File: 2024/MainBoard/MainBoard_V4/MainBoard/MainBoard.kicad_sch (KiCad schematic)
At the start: 96 parts, among them J1 Raspberry_Pi_2_3, J10 ADC3, J11 ADC2, J12 ADC2, J13 Drib, J14 UART, J15 TFT3, J16 CAN_CON, J2 fan, J3 USB_C_Receptacle_USB2.0_16P, J4 CAN_CON, J5 MOLEX MINISPOX, J6 Debug, J7 ADC0, J8 ADC1, J9 ADC2, Q1 NMOS, Q2 PMOS, Q3 PMOS, SW1 SW_MEC_5E, SW2 SW_MEC_5E, SW3 SW_MEC_5E, SW4 SW_Wuerth_450301014042, U1 STM32F446RETx, U2 CH340E, U3 MOUDLE-SEEEDUINO-XIAO, U7 AZ1117-3.3, U8 MAX3051, Y1 CSTNE16M0V530000R0

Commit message: 部品をおいた
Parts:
- J10, J11, J12, J7, J8, J9: footprint Connector_JST:JST_XH_S3B-XH-A_1x03_P2.50mm_Horizontal -> Connector_JST:JST_PH_B3B-PH-K_1x03_P2.00mm_Vertical
- LS1: footprint PKLCS1212E4001-R1:SPKR_PKLCS1212E4001-R1 -> MainBoard:SPKR_PKLCS1212E4001-R1
- ROTSW1: footprint (none) -> Button_Switch_THT:Nidec_Copal_SH-7010C
- U5: footprint Connector_PinHeader_2.54mm:PinHeader_1x05_P2.54mm_Vertical -> Connector_PinHeader_2.54mm:PinHeader_1x04_P2.54mm_Vertical
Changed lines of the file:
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@@
       (effects (font (size 1.27 1.27)))
     )
-    (property "Footprint" "Connector_PinHeader_2.54mm:PinHeader_1x05_P2.54mm_Vertical" (at 222.25 240.03 0)
+    (property "Footprint" "Connector_PinHeader_2.54mm:PinHeader_1x04_P2.54mm_Vertical" (at 222.25 240.03 0)
       (effects (font (size 1.27 1.27)) hide)
     )
@@
       (effects (font (size 1.27 1.27)) (justify left) hide)
     )
-    (property "Footprint" "PKLCS1212E4001-R1:SPKR_PKLCS1212E4001-R1" (at 398.78 52.07 0)
+    (property "Footprint" "MainBoard:SPKR_PKLCS1212E4001-R1" (at 398.78 52.07 0)
       (effects (font (size 1.27 1.27)) (justify bottom) hide)
     )
@@
       (effects (font (size 1.27 1.27)) (justify left))
     )
-    (property "Footprint" "Connector_JST:JST_XH_S3B-XH-A_1x03_P2.50mm_Horizontal" (at 483.87 119.38 0)
+    (property "Footprint" "Connector_JST:JST_PH_B3B-PH-K_1x03_P2.00mm_Vertical" (at 483.87 119.38 0)
       (effects (font (size 1.27 1.27)) hide)
     )
@@
       (effects (font (size 1.27 1.27)) (justify left))
     )
-    (property "Footprint" "Connector_JST:JST_XH_S3B-XH-A_1x03_P2.50mm_Horizontal" (at 483.87 99.06 0)
+    (property "Footprint" "Connector_JST:JST_PH_B3B-PH-K_1x03_P2.00mm_Vertical" (at 483.87 99.06 0)
       (effects (font (size 1.27 1.27)) hide)
     )
@@
       (effects (font (size 1.27 1.27)) (justify left))
     )
-    (property "Footprint" "Connector_JST:JST_XH_S3B-XH-A_1x03_P2.50mm_Horizontal" (at 514.35 119.38 0)
+    (property "Footprint" "Connector_JST:JST_PH_B3B-PH-K_1x03_P2.00mm_Vertical" (at 514.35 119.38 0)
       (effects (font (size 1.27 1.27)) hide)
     )
@@
       (effects (font (size 1.27 1.27)) (justify left))
     )
-    (property "Footprint" "Connector_JST:JST_XH_S3B-XH-A_1x03_P2.50mm_Horizontal" (at 483.87 78.74 0)
+    (property "Footprint" "Connector_JST:JST_PH_B3B-PH-K_1x03_P2.00mm_Vertical" (at 483.87 78.74 0)
       (effects (font (size 1.27 1.27)) hide)
     )
@@
       (effects (font (size 1.27 1.27)))
     )
-    (property "Footprint" "" (at 133.35 237.49 0)
+    (property "Footprint" "Button_Switch_THT:Nidec_Copal_SH-7010C" (at 133.35 237.49 0)
       (effects (font (size 1.27 1.27)) (justify left) hide)
     )
@@
       (effects (font (size 1.27 1.27)) (justify left))
     )
-    (property "Footprint" "Connector_JST:JST_XH_S3B-XH-A_1x03_P2.50mm_Horizontal" (at 514.35 78.74 0)
+    (property "Footprint" "Connector_JST:JST_PH_B3B-PH-K_1x03_P2.00mm_Vertical" (at 514.35 78.74 0)
       (effects (font (size 1.27 1.27)) hide)
     )
@@
       (effects (font (size 1.27 1.27)) (justify left))
     )
-    (property "Footprint" "Connector_JST:JST_XH_S3B-XH-A_1x03_P2.50mm_Horizontal" (at 514.35 99.06 0)
+    (property "Footprint" "Connector_JST:JST_PH_B3B-PH-K_1x03_P2.00mm_Vertical" (at 514.35 99.06 0)
       (effects (font (size 1.27 1.27)) hide)
     )

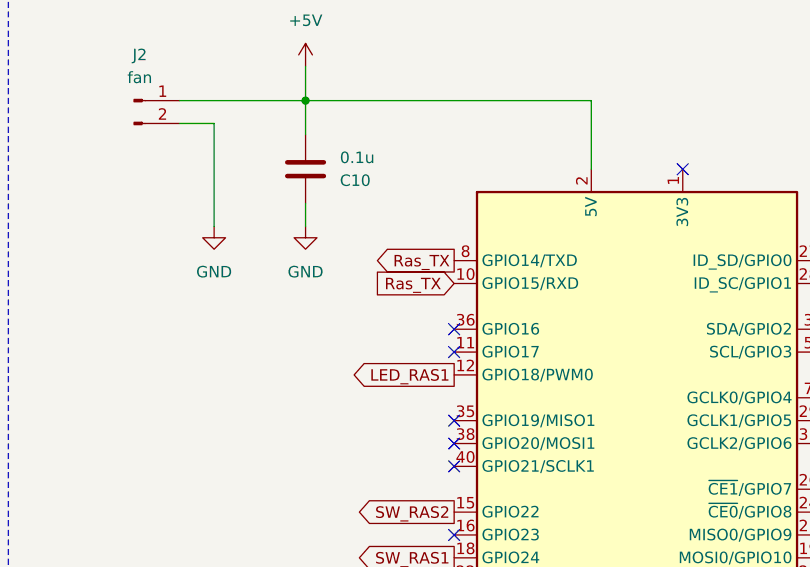
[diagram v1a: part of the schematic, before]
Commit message: わくぎめ
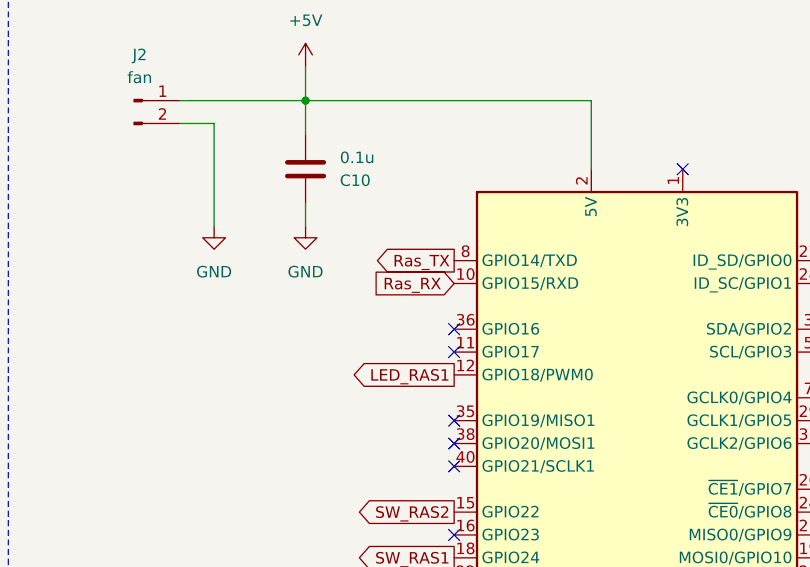
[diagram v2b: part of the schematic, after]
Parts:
- J10, J11, J12, J7, J8, J9: footprint Connector_JST:JST_PH_B3B-PH-K_1x03_P2.00mm_Vertical -> Connector_JST:JST_PH_S3B-PH-K_1x03_P2.00mm_Horizontal
- J5: footprint Connector_Molex:Molex_SPOX_5267-06A_1x06_P2.50mm_Vertical -> Connector_Molex:Molex_SPOX_5268-06A_1x06_P2.50mm_Horizontal
- SW2, SW3: footprint Button_Switch_THT:SW_PUSH_6mm -> MainBoard:SW_SKRPACE010
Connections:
- net Ras_RX: now also J1.10 (GPIO15/RXD)
- net Ras_TX: no longer J1.10 (GPIO15/RXD)
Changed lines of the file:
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@@
     )
   )
-  (global_label "Ras_TX" (shape input) (at 74.93 226.06 180) (fields_autoplaced)
+  (global_label "Ras_RX" (shape input) (at 74.93 226.06 180) (fields_autoplaced)
     (effects (font (size 1.27 1.27)) (justify right))
-    (property "Intersheetrefs" "${INTERSHEET_REFS}" (at 65.5788 226.06 0)
+    (property "Intersheetrefs" "${INTERSHEET_REFS}" (at 65.0506 226.06 0)
       (effects (font (size 1.27 1.27)) (justify right) hide)
     )
@@
       (effects (font (size 1.27 1.27)))
     )
-    (property "Footprint" "Button_Switch_THT:SW_PUSH_6mm" (at 138.43 262.89 0)
+    (property "Footprint" "MainBoard:SW_SKRPACE010" (at 138.43 262.89 0)
       (effects (font (size 1.27 1.27)) hide)
     )
@@
       (effects (font (size 1.27 1.27)) (justify left))
     )
-    (property "Footprint" "Connector_JST:JST_PH_B3B-PH-K_1x03_P2.00mm_Vertical" (at 483.87 119.38 0)
+    (property "Footprint" "Connector_JST:JST_PH_S3B-PH-K_1x03_P2.00mm_Horizontal" (at 483.87 119.38 0)
       (effects (font (size 1.27 1.27)) hide)
     )
@@
       (effects (font (size 1.27 1.27)) (justify left))
     )
-    (property "Footprint" "Connector_Molex:Molex_SPOX_5267-06A_1x06_P2.50mm_Vertical" (at 486.41 55.88 0)
+    (property "Footprint" "Connector_Molex:Molex_SPOX_5268-06A_1x06_P2.50mm_Horizontal" (at 486.41 55.88 0)
       (effects (font (size 1.27 1.27)) hide)
     )
@@
       (effects (font (size 1.27 1.27)) (justify left))
     )
-    (property "Footprint" "Connector_JST:JST_PH_B3B-PH-K_1x03_P2.00mm_Vertical" (at 483.87 99.06 0)
+    (property "Footprint" "Connector_JST:JST_PH_S3B-PH-K_1x03_P2.00mm_Horizontal" (at 483.87 99.06 0)
       (effects (font (size 1.27 1.27)) hide)
     )
@@
       (effects (font (size 1.27 1.27)) (justify left))
     )
-    (property "Footprint" "Connector_JST:JST_PH_B3B-PH-K_1x03_P2.00mm_Vertical" (at 514.35 119.38 0)
+    (property "Footprint" "Connector_JST:JST_PH_S3B-PH-K_1x03_P2.00mm_Horizontal" (at 514.35 119.38 0)
       (effects (font (size 1.27 1.27)) hide)
     )
@@
       (effects (font (size 1.27 1.27)) (justify left))
     )
-    (property "Footprint" "Connector_JST:JST_PH_B3B-PH-K_1x03_P2.00mm_Vertical" (at 483.87 78.74 0)
+    (property "Footprint" "Connector_JST:JST_PH_S3B-PH-K_1x03_P2.00mm_Horizontal" (at 483.87 78.74 0)
       (effects (font (size 1.27 1.27)) hide)
     )
@@
       (effects (font (size 1.27 1.27)) (justify left))
     )
-    (property "Footprint" "Connector_JST:JST_PH_B3B-PH-K_1x03_P2.00mm_Vertical" (at 514.35 78.74 0)
+    (property "Footprint" "Connector_JST:JST_PH_S3B-PH-K_1x03_P2.00mm_Horizontal" (at 514.35 78.74 0)
       (effects (font (size 1.27 1.27)) hide)
     )
@@
       (effects (font (size 1.27 1.27)) (justify left))
     )
-    (property "Footprint" "Connector_JST:JST_PH_B3B-PH-K_1x03_P2.00mm_Vertical" (at 514.35 99.06 0)
+    (property "Footprint" "Connector_JST:JST_PH_S3B-PH-K_1x03_P2.00mm_Horizontal" (at 514.35 99.06 0)
       (effects (font (size 1.27 1.27)) hide)
     )
@@
       (effects (font (size 1.27 1.27)))
     )
-    (property "Footprint" "Button_Switch_THT:SW_PUSH_6mm" (at 138.43 246.38 0)
+    (property "Footprint" "MainBoard:SW_SKRPACE010" (at 138.43 246.38 0)
       (effects (font (size 1.27 1.27)) hide)
     )

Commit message: 途中経過
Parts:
- D5: footprint Diode_THT:D_DO-35_SOD27_P7.62mm_Horizontal -> Diode_SMD:D_SOD-123
- Q2, Q3: footprint (none) -> Package_TO_SOT_SMD:SOT-23
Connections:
- net UART_RX is gone; now on net UART1_TX: J6.1 (Pin_1)
- net UART_TX is gone; now on net UART1_RX: J6.2 (Pin_2)
- net VDD is gone; now on net +3.3V: J6.6 (Pin_6)
- net CANH: now also J16.2 (Pin_2); no longer J16.1 (Pin_1)
- net CANL: now also J16.1 (Pin_1); no longer J16.2 (Pin_2)
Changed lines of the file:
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@@
+    )
+  )
+  (global_label "CANH" (shape bidirectional) (at 509.27 50.8 180) (fields_autoplaced)
+    (effects (font (size 1.27 1.27)) (justify right))
+    (property "Intersheetrefs" "${INTERSHEET_REFS}" (at 500.1539 50.8 0)
+      (effects (font (size 1.27 1.27)) (justify right) hide)
     )
   )
@@
     )
   )
-  (global_label "UART_RX" (shape input) (at 45.72 139.7 0) (fields_autoplaced)
-    (effects (font (size 1.27 1.27)) (justify left))
-    (property "Intersheetrefs" "${INTERSHEET_REFS}" (at 56.1692 139.7 0)
-      (effects (font (size 1.27 1.27)) (justify left) hide)
-    )
-  )
   (global_label "LED_RAS1" (shape output) (at 495.3 184.15 180) (fields_autoplaced)
     (effects (font (size 1.27 1.27)) (justify right))
@@
     )
   )
-  (global_label "CANH" (shape bidirectional) (at 509.27 48.26 180) (fields_autoplaced)
-    (effects (font (size 1.27 1.27)) (justify right))
-    (property "Intersheetrefs" "${INTERSHEET_REFS}" (at 500.1539 48.26 0)
-      (effects (font (size 1.27 1.27)) (justify right) hide)
-    )
-  )
   (global_label "LED1" (shape output) (at 533.4 171.45 180) (fields_autoplaced)
     (effects (font (size 1.27 1.27)) (justify right))
@@
     )
   )
-  (global_label "UART_TX" (shape output) (at 45.72 142.24 0) (fields_autoplaced)
-    (effects (font (size 1.27 1.27)) (justify left))
-    (property "Intersheetrefs" "${INTERSHEET_REFS}" (at 56.1692 142.24 0)
-      (effects (font (size 1.27 1.27)) (justify left) hide)
-    )
-  )
   (global_label "CANL" (shape bidirectional) (at 509.27 60.96 180) (fields_autoplaced)
     (effects (font (size 1.27 1.27)) (justify right))
@@
     )
   )
-  (global_label "CANL" (shape bidirectional) (at 509.27 50.8 180) (fields_autoplaced)
-    (effects (font (size 1.27 1.27)) (justify right))
-    (property "Intersheetrefs" "${INTERSHEET_REFS}" (at 500.4563 50.8 0)
-      (effects (font (size 1.27 1.27)) (justify right) hide)
-    )
-  )
   (global_label "I2C_SCL" (shape bidirectional) (at 293.37 132.08 180) (fields_autoplaced)
     (effects (font (size 1.27 1.27)) (justify right))
@@
     )
   )
+  (global_label "USB_RX" (shape input) (at 45.72 139.7 0) (fields_autoplaced)
+    (effects (font (size 1.27 1.27)) (justify left))
+    (property "Intersheetrefs" "${INTERSHEET_REFS}" (at 55.0712 139.7 0)
+      (effects (font (size 1.27 1.27)) (justify left) hide)
+    )
+  )
+  (global_label "USB_TX" (shape output) (at 45.72 142.24 0) (fields_autoplaced)
+    (effects (font (size 1.27 1.27)) (justify left))
+    (property "Intersheetrefs" "${INTERSHEET_REFS}" (at 55.0712 142.24 0)
+      (effects (font (size 1.27 1.27)) (justify left) hide)
+    )
+  )
   (global_label "UART4_TX" (shape output) (at 203.2 35.56 180) (fields_autoplaced)
     (effects (font (size 1.27 1.27)) (justify right))
@@
     )
   )
+  (global_label "CANL" (shape bidirectional) (at 509.27 48.26 180) (fields_autoplaced)
+    (effects (font (size 1.27 1.27)) (justify right))
+    (property "Intersheetrefs" "${INTERSHEET_REFS}" (at 500.4563 48.26 0)
+      (effects (font (size 1.27 1.27)) (justify right) hide)
+    )
+  )
   (global_label "RAS_AUDIO" (shape output) (at 115.57 266.7 0) (fields_autoplaced)
     (effects (font (size 1.27 1.27)) (justify left))
@@
       (effects (font (size 1.27 1.27)))
     )
-    (property "Footprint" "" (at 191.77 69.85 0)
+    (property "Footprint" "Package_TO_SOT_SMD:SOT-23" (at 191.77 69.85 0)
       (effects (font (size 1.27 1.27)) hide)
     )
@@
     )
   )
-  (symbol (lib_id "power:VDD") (at 58.42 139.7 0) (unit 1)
-    (in_bom yes) (on_board yes) (dnp no)
-    (property "Reference" "#PWR064" (at 58.42 143.51 0)
-      (effects (font (size 1.27 1.27)) hide)
-    )
-    (property "Value" "VDD" (at 58.801 136.4488 0)
-      (effects (font (size 1.27 1.27)) (justify left))
-    )
-    (property "Footprint" "" (at 58.42 139.7 0)
-      (effects (font (size 1.27 1.27)) hide)
-    )
-    (property "Datasheet" "" (at 58.42 139.7 0)
-      (effects (font (size 1.27 1.27)) hide)
-    )
-    (pin "1")
-    (instances
-      (project "MainBoard"
-        (path "/0f1369eb-a284-48b8-a3ed-798a8062c1cf"
-          (reference "#PWR064") (unit 1)
-        )
-      )
-    )
-  )
   (symbol (lib_id "Device:LED") (at 527.05 201.93 90) (unit 1)
     (in_bom yes) (on_board yes) (dnp no)
@@
       (effects (font (size 1.27 1.27)))
     )
-    (property "Footprint" "" (at 186.69 69.85 0)
+    (property "Footprint" "Package_TO_SOT_SMD:SOT-23" (at 186.69 69.85 0)
       (effects (font (size 1.27 1.27)) hide)
     )
@@
     )
   )
+  (symbol (lib_id "power:+3.3V") (at 58.42 139.7 0) (unit 1)
+    (in_bom yes) (on_board yes) (dnp no) (fields_autoplaced)
+    (property "Reference" "#PWR064" (at 58.42 143.51 0)
+      (effects (font (size 1.27 1.27)) hide)
+    )
+    (property "Value" "+3.3V" (at 58.42 134.62 0)
+      (effects (font (size 1.27 1.27)))
+    )
+    (property "Footprint" "" (at 58.42 139.7 0)
+      (effects (font (size 1.27 1.27)) hide)
+    )
+    (property "Datasheet" "" (at 58.42 139.7 0)
+      (effects (font (size 1.27 1.27)) hide)
+    )
+    (pin "1")
+    (instances
+      (project "MainBoard"
+        (path "/0f1369eb-a284-48b8-a3ed-798a8062c1cf"
+          (reference "#PWR064") (unit 1)
+        )
+      )
+    )
+  )
   (symbol (lib_id "Switch:SW_Wuerth_450301014042") (at 49.53 74.93 180) (unit 1)
     (in_bom yes) (on_board yes) (dnp no)
@@
       (effects (font (size 1.27 1.27)))
     )
-    (property "Footprint" "Diode_THT:D_DO-35_SOD27_P7.62mm_Horizontal" (at 381 69.85 0)
-      (effects (font (size 1.27 1.27)) hide)
-    )
+    (property "Footprint" "Diode_SMD:D_SOD-123" (at 381 69.85 0)
+      (effects (font (size 1.27 1.27)) hide)
+    )
